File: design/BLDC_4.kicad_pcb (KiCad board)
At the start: 4 copper layers, 38.5 x 65 mm, 127 parts, among them K1 SERVO, P1 HALL/Encoder, P101 CANBUS, P2 SWD, P3 PWR_COMM, P4 IN+, P5 IN-, P6 MOTOR1, P7 MOTOR2, P9 MOTOR3, Q1 IRFS7530, Q2 IRFS7530, Q3 IRFS7530, Q4 IRFS7530, Q5 IRFS7530, Q6 IRFS7530, U1 STM32F40X_LQFP64, U2 TC2117, U3 DRV8302, U401 SN65HVD232, X1 MINI-USB-SHIELD-32005-201, X2 8MHz 10ppm

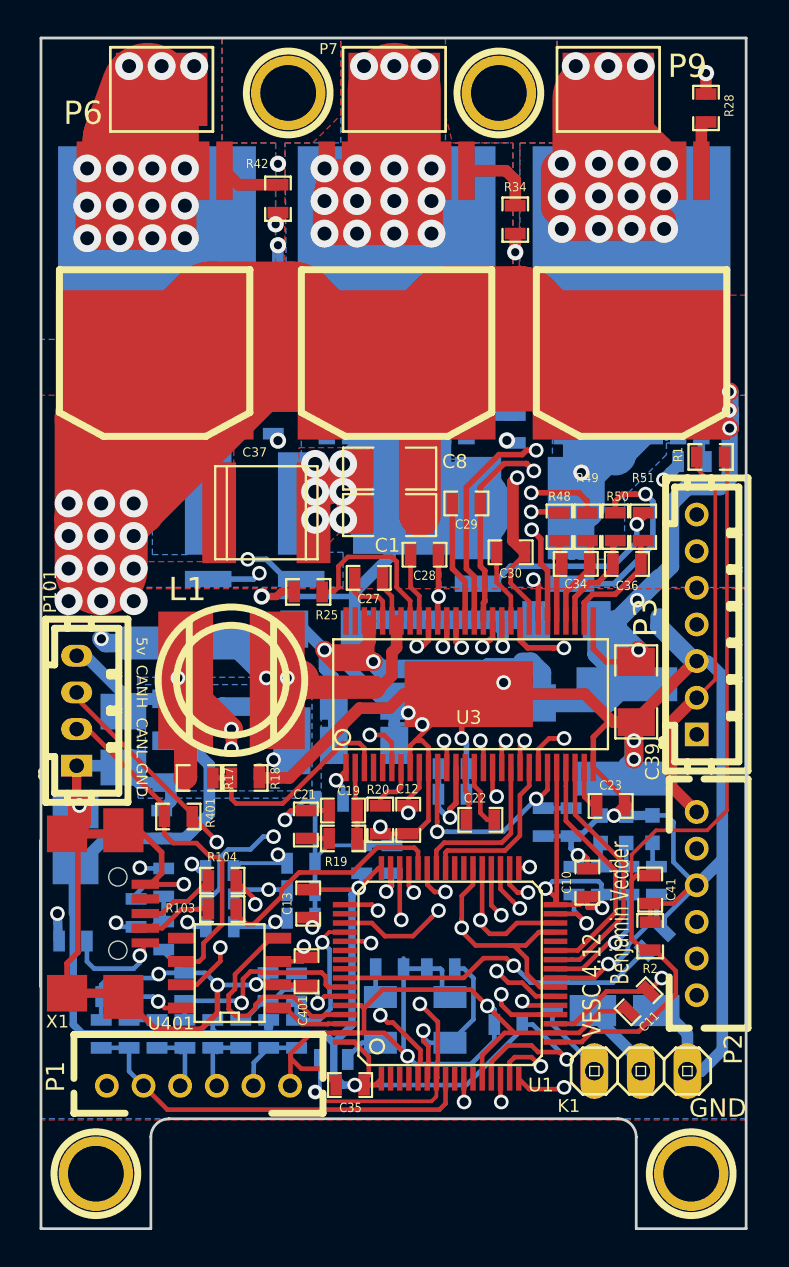
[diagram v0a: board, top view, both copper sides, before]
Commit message: fork
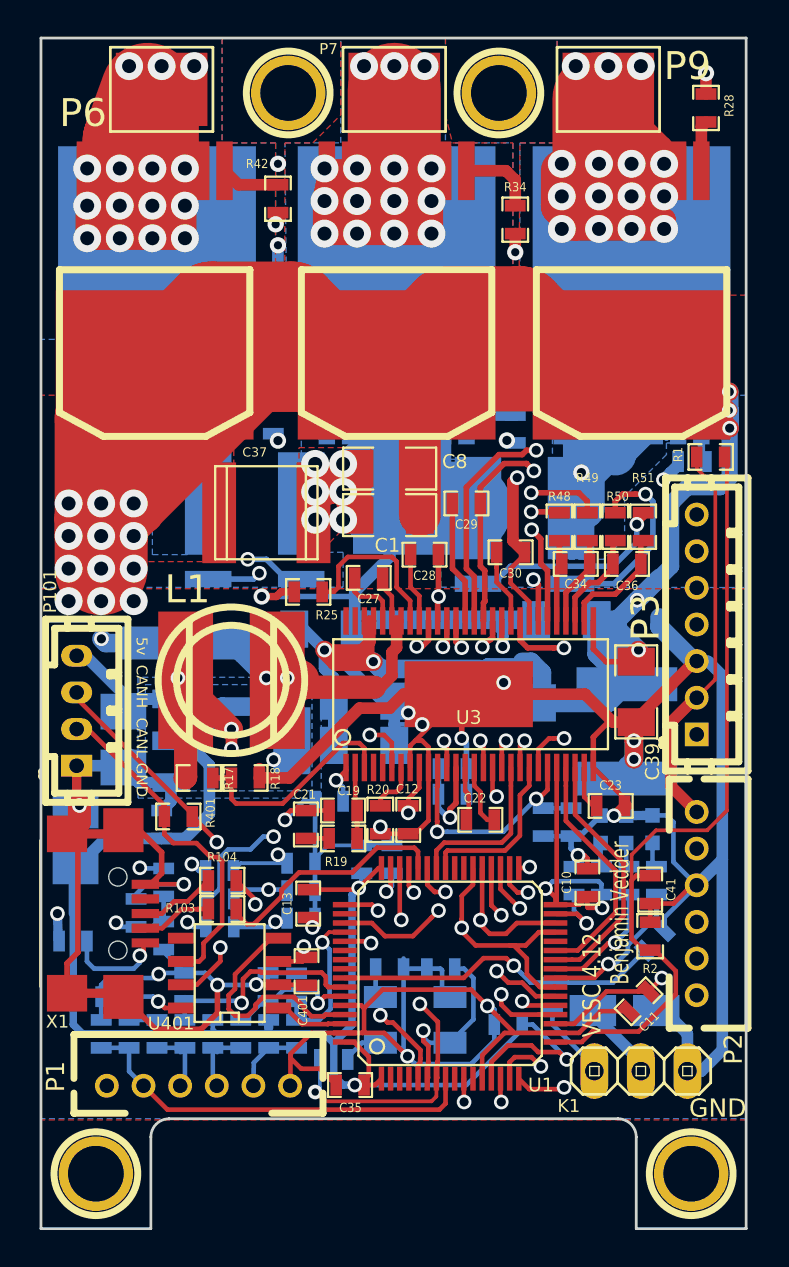
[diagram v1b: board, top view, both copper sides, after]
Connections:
- net /MCU/MISO_ADC_EXT2 renamed /MISO_RX_SCL
- net /MCU/RX_SCL_MOSI renamed /RX_SCL_MOSI
- net /MCU/SCK_ADC_EXT renamed /SCK_ADC_EXT
- net /MCU/TX_SDA_NSS renamed /TX_SDA
